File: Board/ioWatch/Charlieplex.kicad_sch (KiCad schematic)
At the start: 72 parts

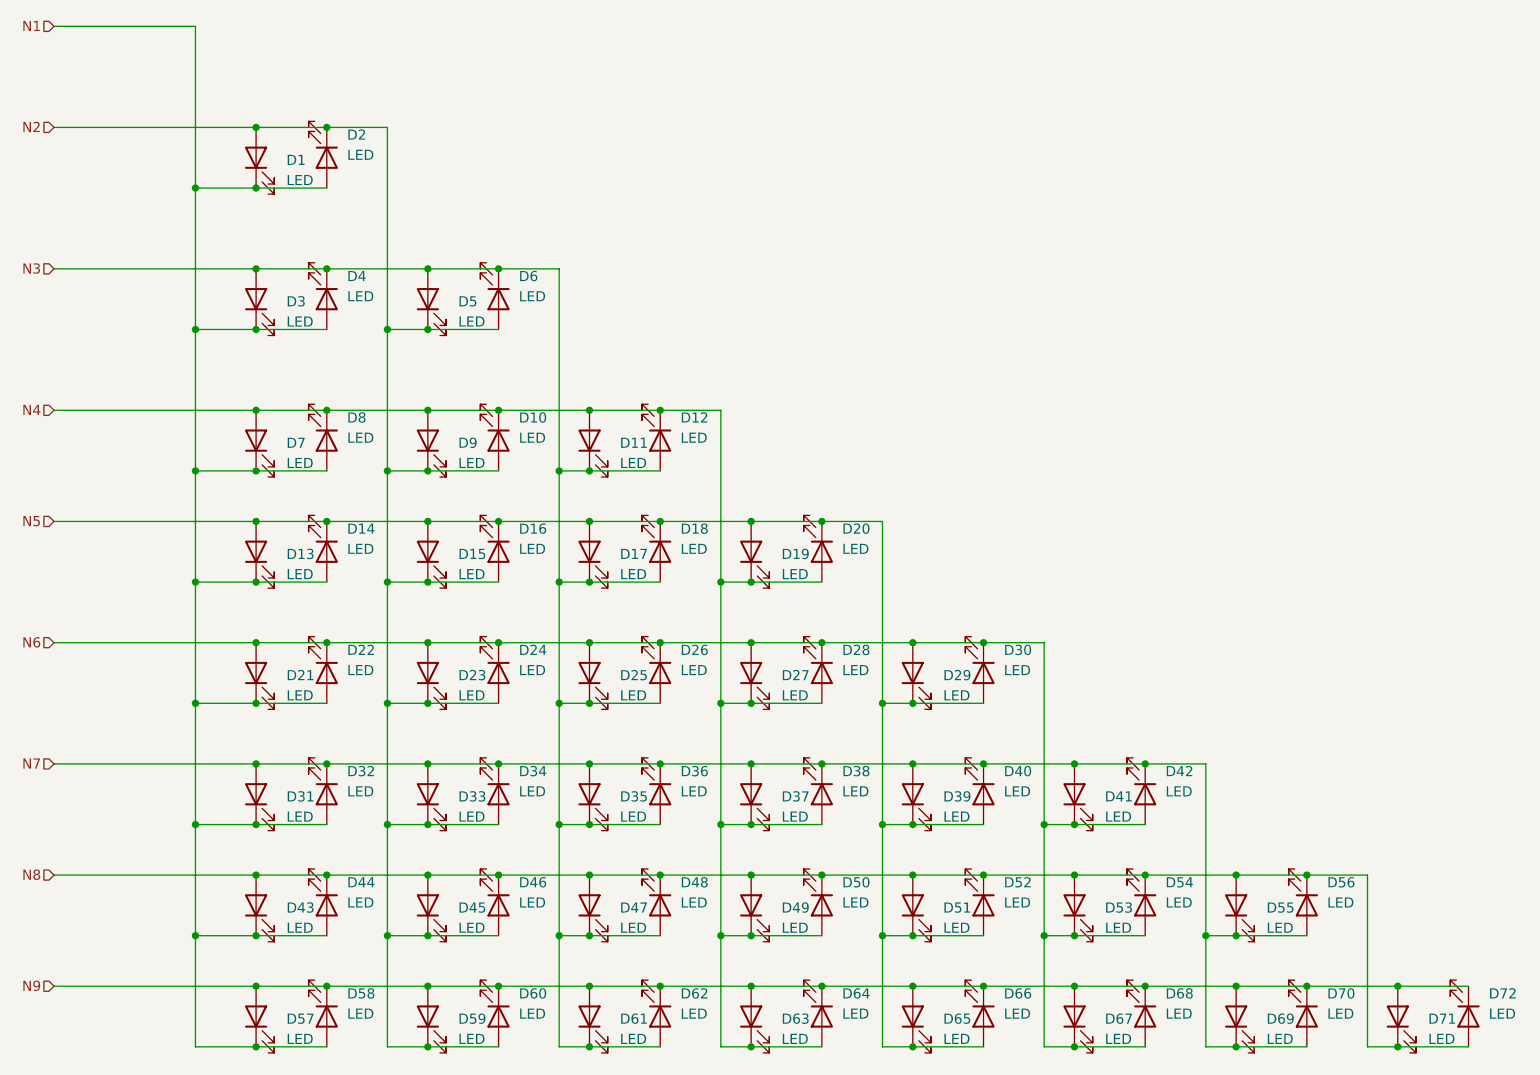
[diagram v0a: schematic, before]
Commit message: work
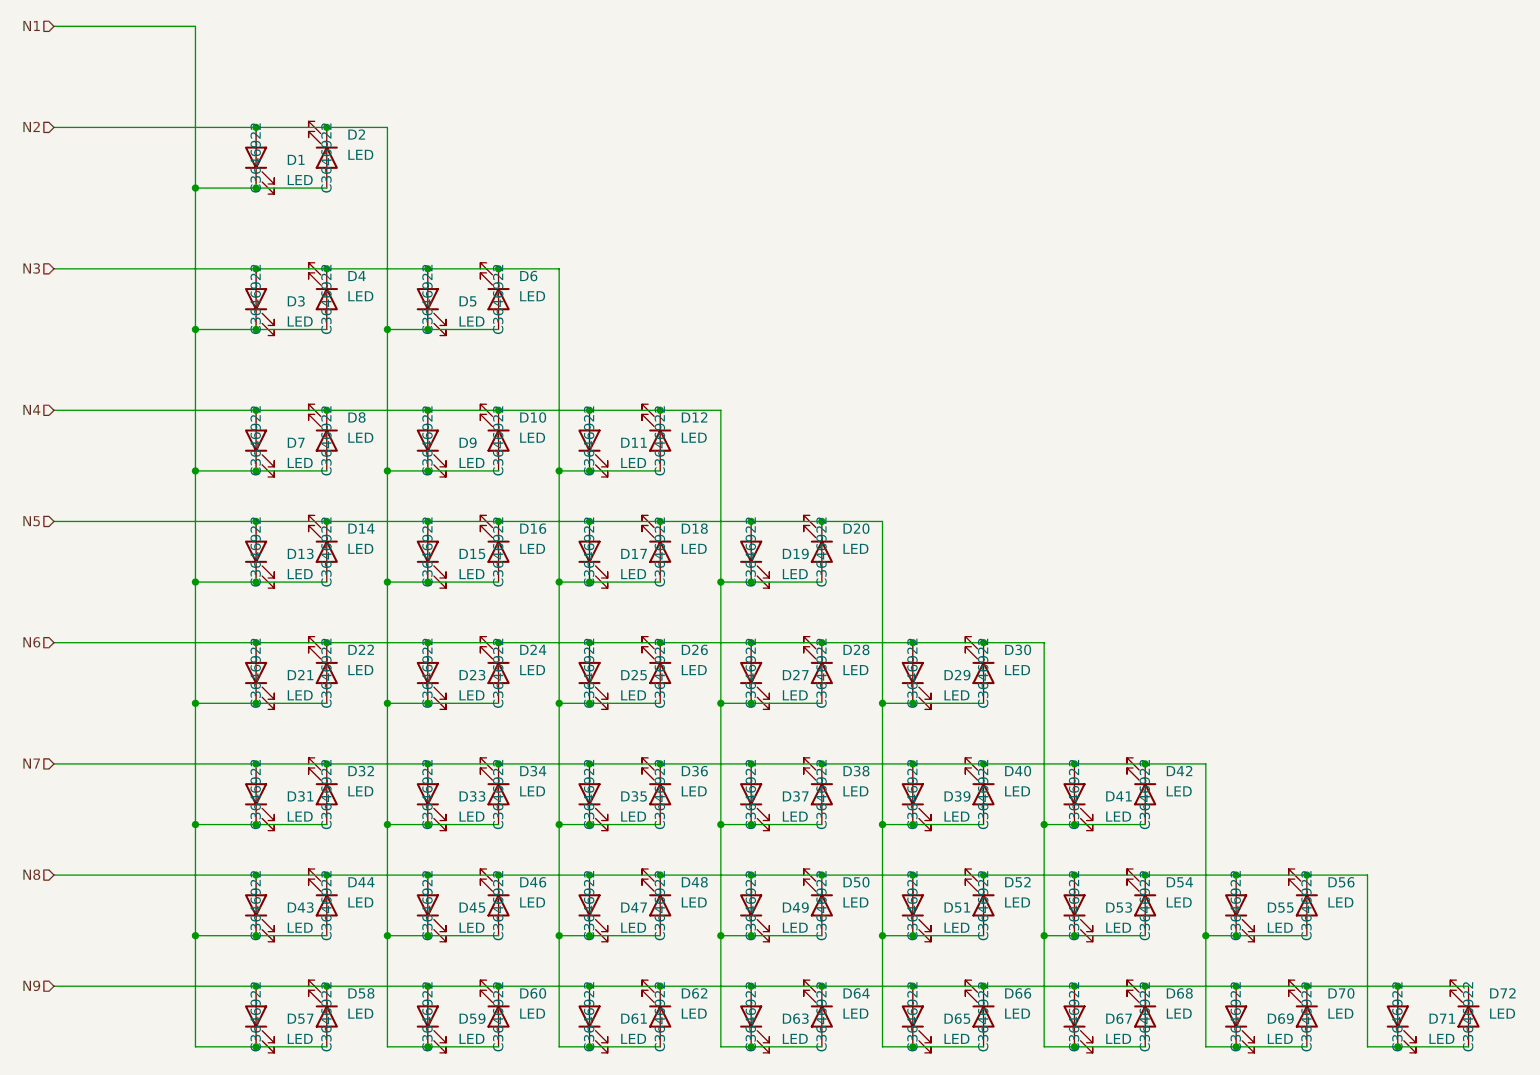
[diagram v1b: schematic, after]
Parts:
- D1, D10, D11, D12, D13, D14, D15, D16, D17, D18, D19, D2, D20, D21, D22, D23, D24, D25, D26, D27, D28, D29, D3, D30, D31, D32, D33, D34, D35, D36, D37, D38, D39, D4, D40, D41, D42, D43, D44, D45, D46, D47, D48, D49, D5, D50, D51, D52, D53, D54, D55, D56, D57, D58, D59, D6, D60, D61, D62, D63, D64, D65, D66, D67, D68, D69, D7, D70, D71, D72, D8, D9: LCSC (none) -> C3646922
